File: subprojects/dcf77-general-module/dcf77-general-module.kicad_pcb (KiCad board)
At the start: 2 copper layers, 22.1 x 14.2 mm, 2 parts

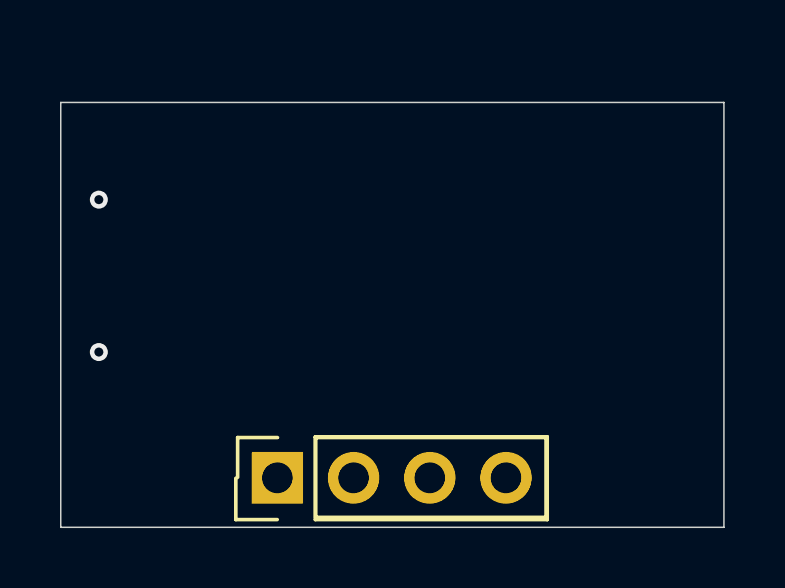
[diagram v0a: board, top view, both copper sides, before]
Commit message: preventivne
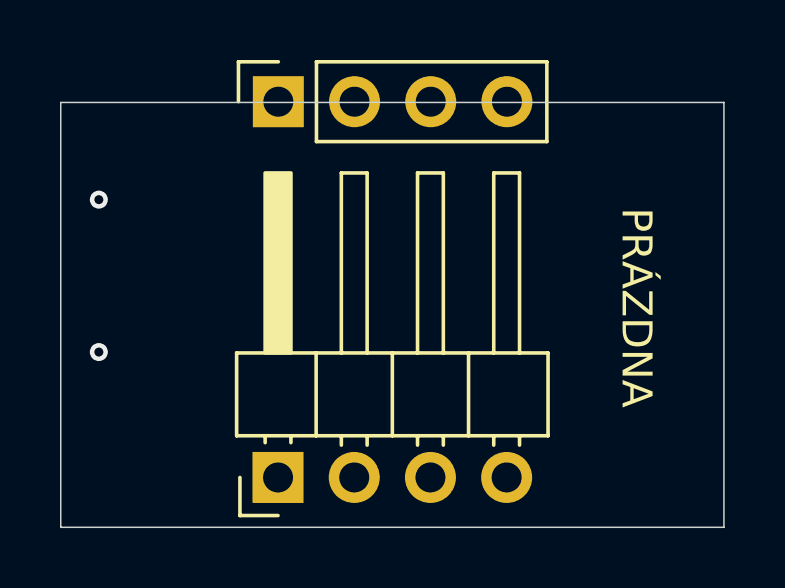
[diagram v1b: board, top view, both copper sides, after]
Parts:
- removed the REF** at (111.6, 88.0)
- added REF**: PinHeader_1x04_P2.54mm_Horizontal, Connector_PinHeader_2.54mm:PinHeader_1x04_P2.54mm_Horizontal, F.Cu at (111.6, 88.0)
- moved REF** 12.5 mm to (111.6, 75.5)
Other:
- board text added: "PRÁZDNA"
- board text added: "STRANA SÚČIASTOK"
